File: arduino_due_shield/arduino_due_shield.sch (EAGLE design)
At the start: 27 parts, among them J12 ARDUINO_MEGA_R3FULL, J13 POLOLU-2595, J14 POLOLU-2807, J15 POLOLU-2595

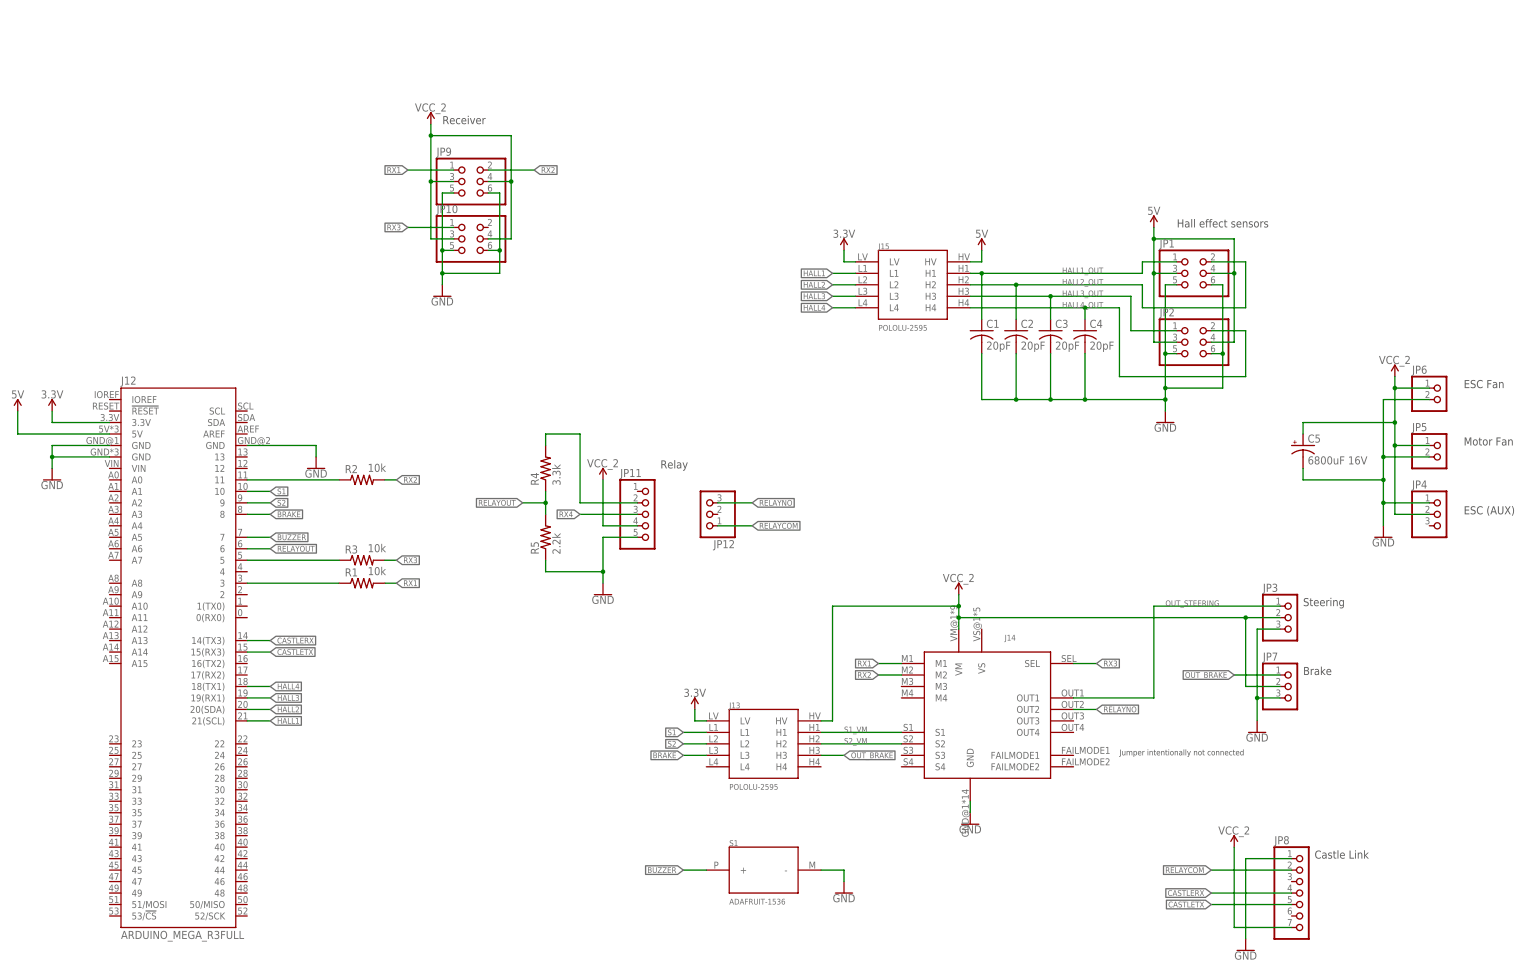
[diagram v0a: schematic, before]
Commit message: Finish schematic and PCB design
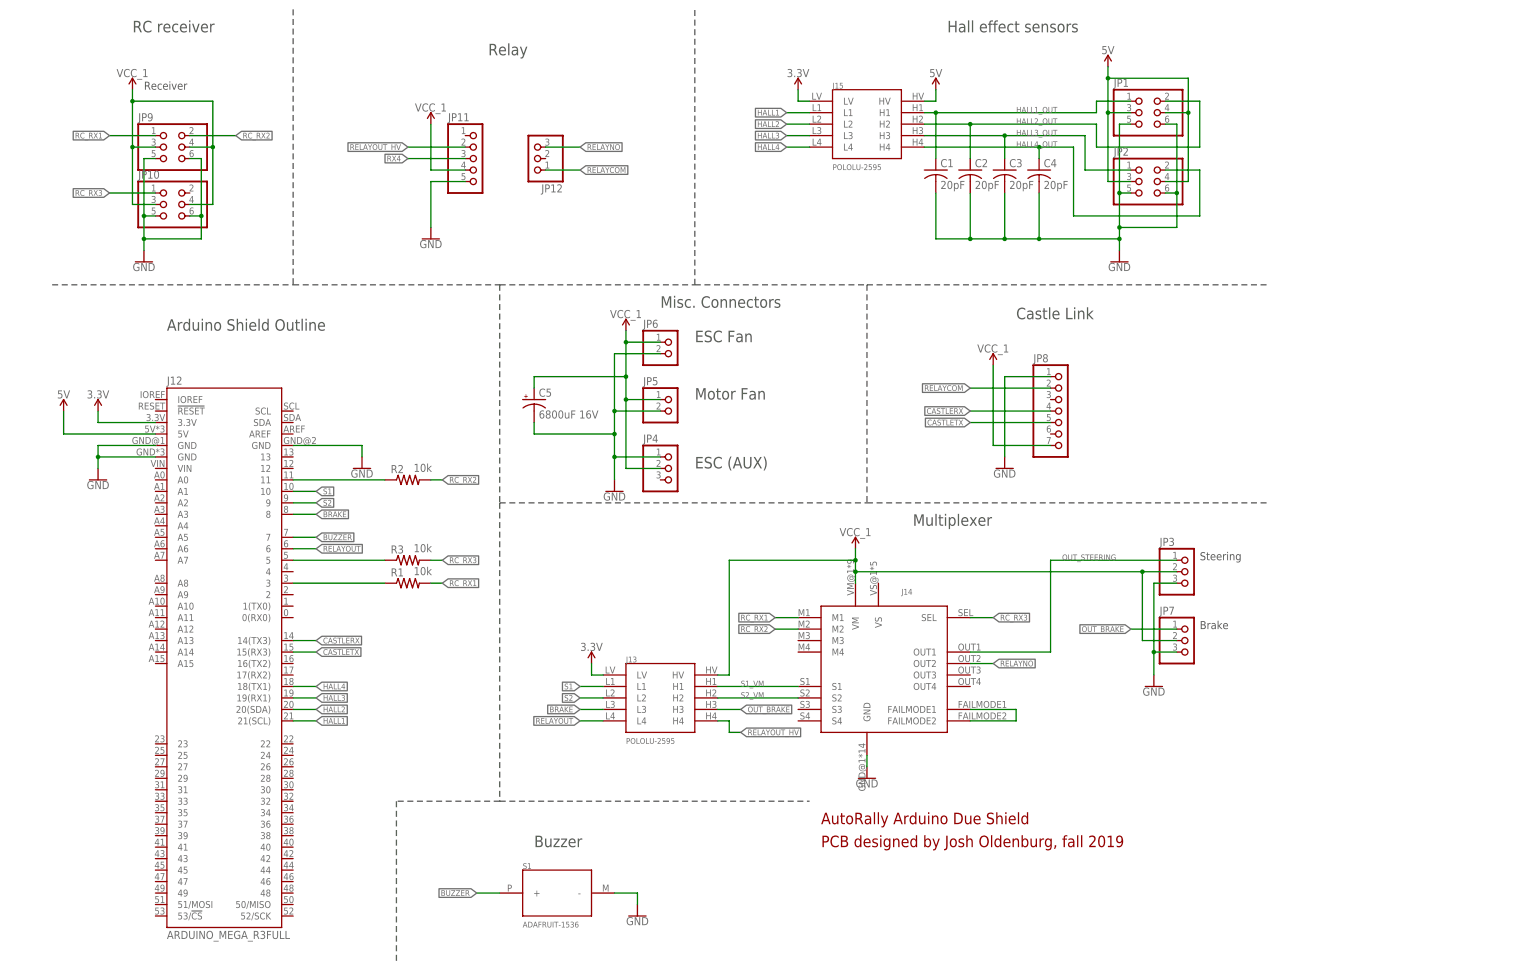
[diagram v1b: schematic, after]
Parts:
- removed R4: 3.3k, resistor:R-US_0204/7
- removed R5: 2.2k, resistor:R-US_0204/7
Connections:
- net RX1 renamed RC_RX1
- net RX2 renamed RC_RX2
- net RX3 renamed RC_RX3
- removed net RELAYHV: JP11.2, R4.2
- new net N$2: J14.FAILMODE1, J14.FAILMODE2
- new net RELAYOUT_HV: J13.H4, JP11.2
- net GND: no longer R5.1
- net RELAYOUT: now also J13.L4; no longer R4.1, R5.2
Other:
- note added: "Arduino Shield Outline"
- note added: "AutoRally Arduino Due Shield"
- note added: "Buzzer"
- note added: "Misc. Connectors"
- note added: "Multiplexer"
- note added: "PCB designed by Josh Oldenburg, fall 2019"
- note added: "RC receiver"
- note removed: "Jumper intentionally not connected"
- moved on the sheet: C1, C2, C3, C4, C5, J12, J13, J14, J15, JP1, JP10, JP11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
